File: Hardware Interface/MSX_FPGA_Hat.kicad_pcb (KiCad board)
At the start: 2 copper layers, 99.9 x 64 mm, 41 parts, among them J1 Conn_01x03_Female, J2 SND, J3 AudioJack3, J4 /CS12, Q1 2N3904, Q2 2N3904, SW1 RESET, U1 74LVC245, U2 74LVC245, U3 74LVC245, U4 74LVC245, U5 74LVC245, U6 LM1117-3.3

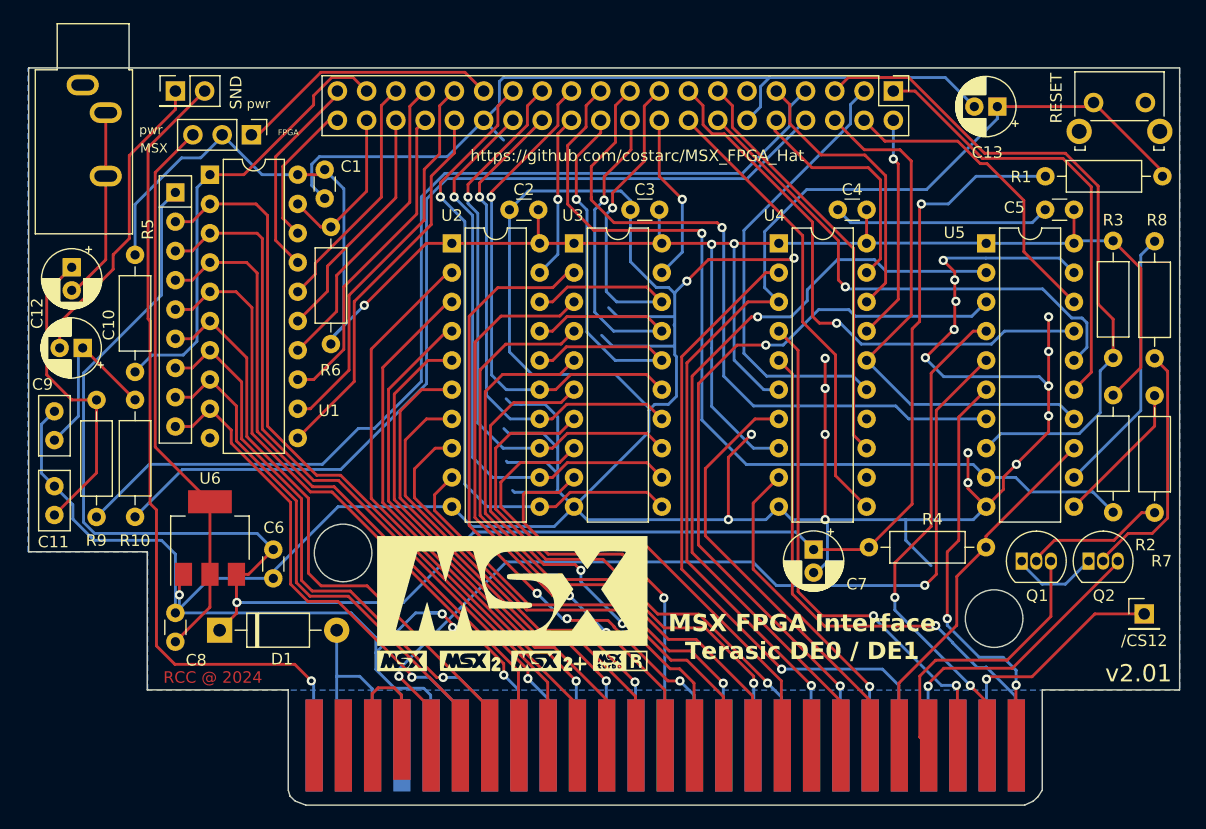
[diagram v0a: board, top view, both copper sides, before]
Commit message: V2.01
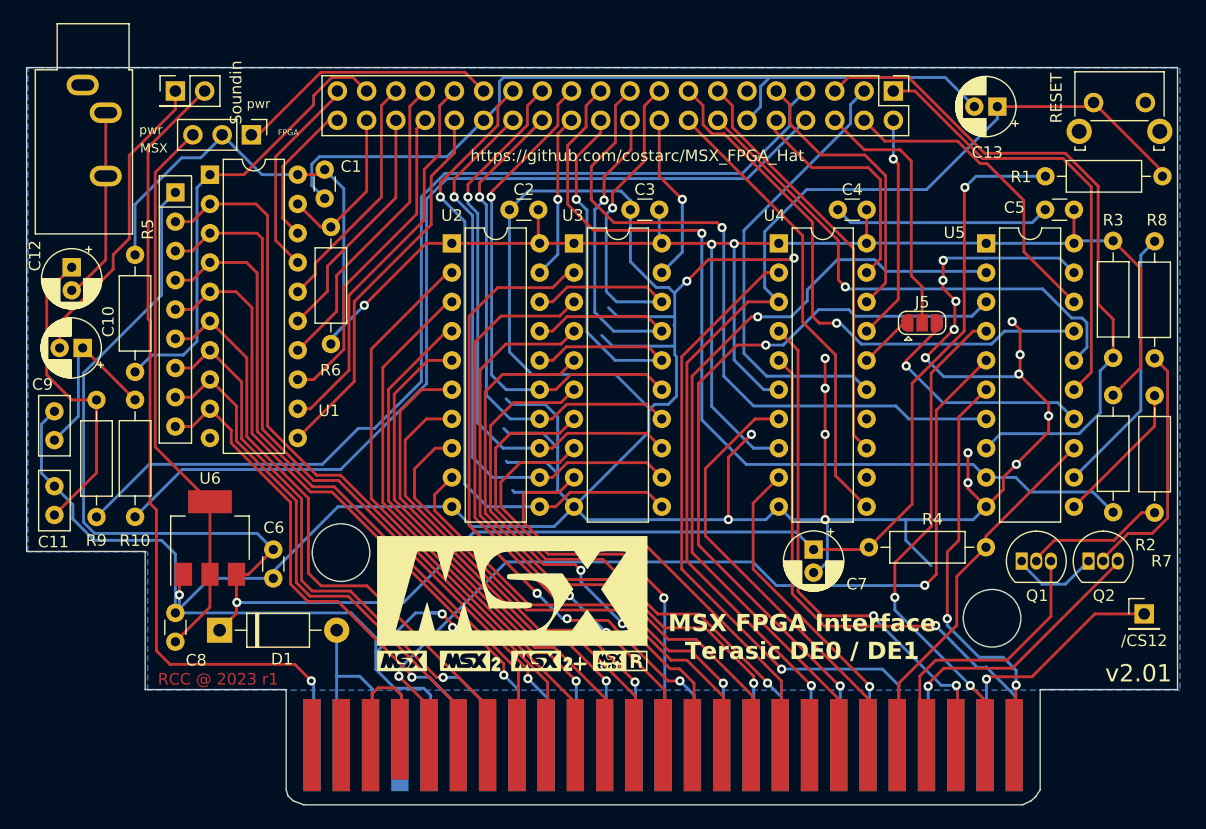
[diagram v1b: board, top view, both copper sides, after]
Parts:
- added J5: RFSH_CS2, Jumper:SolderJumper-3_P1.3mm_Open_RoundedPad1.0x1.5mm, F.Cu at (127.9, 46.7)
- J2: value SND -> Soundin
- moved CONN1 0.18 mm to (99.1, 53.1)
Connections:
- U4 pad 16: /C_CS2_RFSH -> /C_RFSH
- U5 pad 14: /C_CS2_RFSH -> /C_CS2
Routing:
- net /C_CS2_RFSH: track 47.8 -> 22.7 mm
- net /C_CS2: track 0.00 -> 22.3 mm, vias 0 -> 1
- net /C_RFSH: track 0.00 -> 4.92 mm
- net GNDREF: track 468.0 -> 463.8 mm
- net Vcc: track 160.7 -> 159.3 mm
